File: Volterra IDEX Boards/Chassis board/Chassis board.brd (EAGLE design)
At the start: 102.2 x 54 mm, 29 parts, among them K1 FFC/FPC/34PIN/1MMPITCH/TOPLOCK, K2 FFC/FPC/34PIN/1MMPITCH/TOPLOCK, K3 FFC/FPC/34PIN/1MMPITCH/TOPLOCK, X1 JST-XH-02-PIN-LONG-PAD

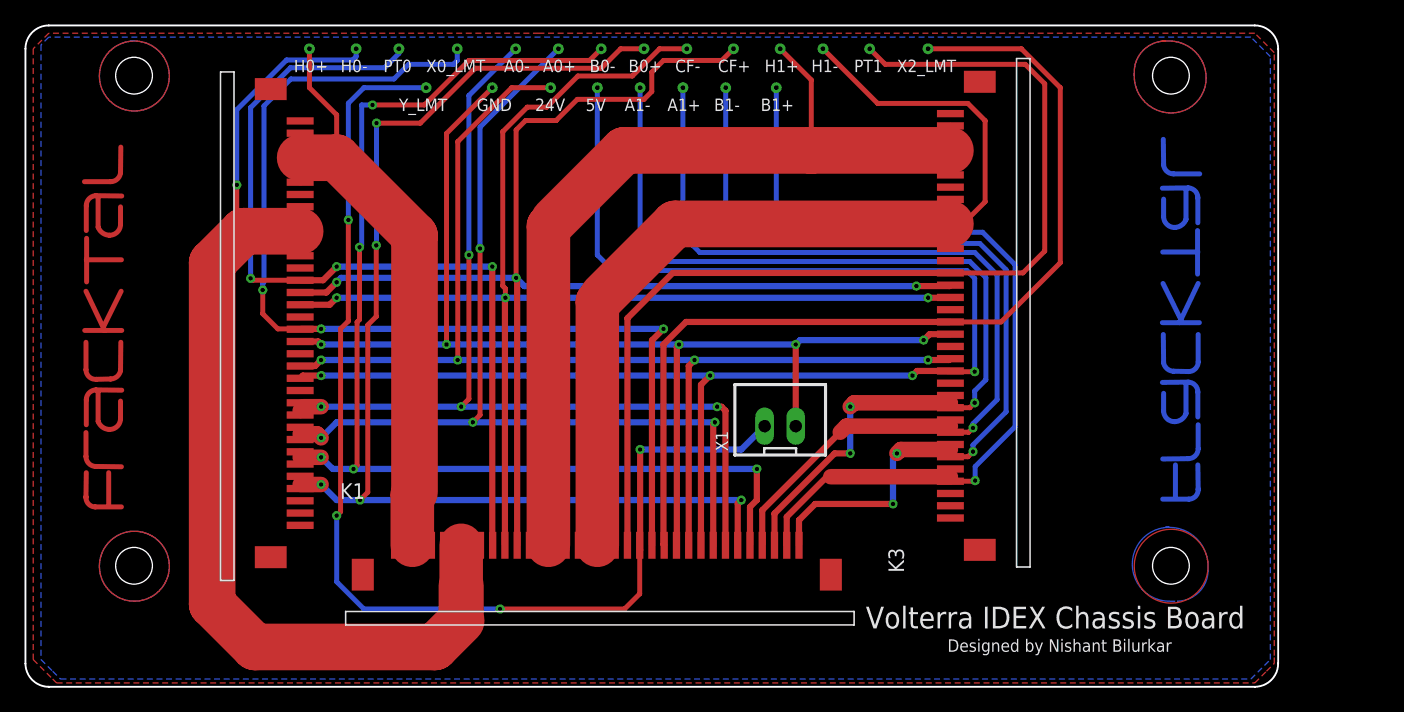
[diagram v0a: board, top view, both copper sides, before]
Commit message: DRC checked of Chassis, Carriage 1 & 2, and created CAM files
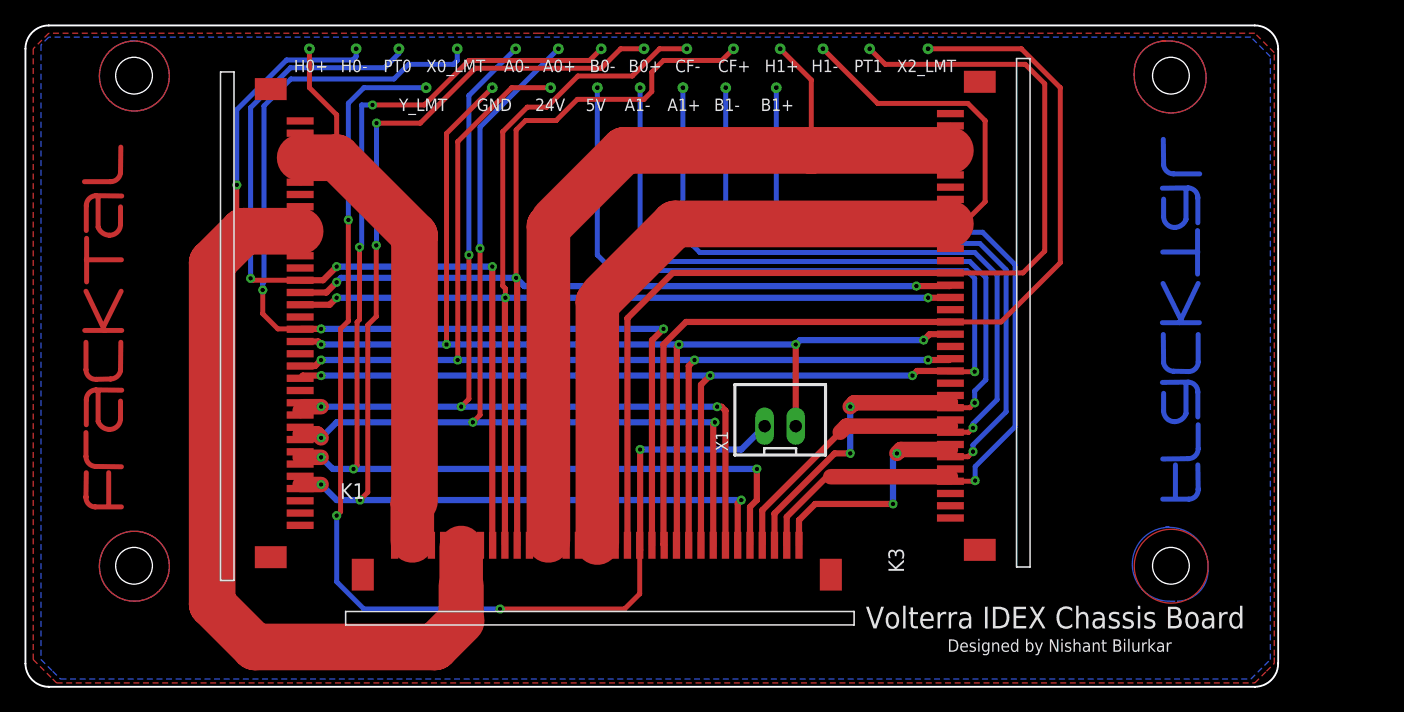
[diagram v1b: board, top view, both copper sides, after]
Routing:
- net H0+: track 53.9 -> 55.4 mm
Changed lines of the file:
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@@
 <contactref element="K2" pad="6"/>
 <contactref element="TP21" pad="P$1"/>
-<wire x1="37.7505" y1="15.3595" x2="38.7505" y2="15.3595" width="0.1524" layer="1"/>
-<wire x1="38.7505" y1="15.3595" x2="39.1922" y2="15.3595" width="0.1524" layer="1"/>
-<wire x1="39.37" y1="15.3595" x2="39.7505" y2="15.3595" width="0.1524" layer="1"/>
-<wire x1="39.7505" y1="15.3595" x2="40.7505" y2="15.3595" width="0.1524" layer="1"/>
-<wire x1="39.1922" y1="19.5072" x2="39.37" y2="19.685" width="3.556" layer="1"/>
-<wire x1="39.1922" y1="19.5072" x2="39.1922" y2="15.3595" width="3.556" layer="1"/>
-<wire x1="39.37" y1="19.685" x2="39.37" y2="40.64" width="3.81" layer="1"/>
+<wire x1="39.1922" y1="18.796" x2="39.37" y2="18.9738" width="3.556" layer="1"/>
+<wire x1="39.1922" y1="15.7151" x2="39.1922" y2="18.796" width="3.556" layer="1"/>
+<wire x1="39.37" y1="18.9738" x2="39.37" y2="40.64" width="3.81" layer="1"/>
 <wire x1="30.04" y1="46.99" x2="33.02" y2="46.99" width="3.81" layer="1"/>
 <wire x1="39.37" y1="40.64" x2="33.02" y2="46.99" width="3.81" layer="1"/>
@@
 <wire x1="30.04" y1="46.99" x2="30.04" y2="45.99" width="0.508" layer="1"/>
 <wire x1="30.04" y1="45.99" x2="30.04" y2="44.99" width="0.508" layer="1"/>
+<wire x1="40.7505" y1="15.3595" x2="39.7505" y2="15.3595" width="0.2032" layer="1"/>
+<wire x1="37.7505" y1="15.3595" x2="38.7505" y2="15.3595" width="0.2032" layer="1"/>
+<wire x1="38.7505" y1="15.3595" x2="39.7505" y2="15.3595" width="0.2032" layer="1"/>
+<wire x1="37.7505" y1="15.3595" x2="38.1061" y2="15.7151" width="0.2032" layer="1"/>
+<wire x1="38.1061" y1="15.7151" x2="39.1922" y2="15.7151" width="0.2032" layer="1"/>
 </signal>
 <signal name="H0-">
@@
 <contactref element="K2" pad="11"/>
 <contactref element="TP1" pad="P$1"/>
-<wire x1="41.7505" y1="15.3595" x2="42.7505" y2="15.3595" width="0.1524" layer="1"/>
-<wire x1="43.7505" y1="15.3595" x2="43.18" y2="15.3595" width="0.1524" layer="1"/>
-<wire x1="42.7505" y1="15.3595" x2="43.18" y2="15.3595" width="0.1524" layer="1"/>
-<wire x1="43.7505" y1="15.3595" x2="44.7505" y2="15.3595" width="0.1524" layer="1"/>
-<wire x1="43.18" y1="15.3595" x2="43.18" y2="12.065" width="3.556" layer="1"/>
+<wire x1="43.18" y1="12.065" x2="43.18" y2="15.1817" width="3.556" layer="1"/>
 <wire x1="43.18" y1="12.065" x2="43.18" y2="9.2075" width="3.683" layer="1"/>
 <wire x1="43.18" y1="9.2075" x2="41.0337" y2="7.0612" width="3.81" layer="1"/>
@@
 <wire x1="30.04" y1="40.99" x2="30.04" y2="39.99" width="1.27" layer="1"/>
 <wire x1="30.04" y1="41.99" x2="30.04" y2="42.99" width="0.508" layer="1"/>
-<wire x1="30.04" y1="39.99" x2="30.04" y2="38.99" width="0.1524" layer="1"/>
 <wire x1="25.4325" y1="40.99" x2="24.8666" y2="41.5559" width="0.4064" layer="1"/>
 <wire x1="24.8666" y1="41.5559" x2="24.8666" y2="44.7675" width="0.4064" layer="1"/>
@@
 <wire x1="34.3281" y1="54.9656" x2="34.6075" y2="55.245" width="0.4064" layer="16"/>
 <wire x1="34.6075" y1="55.245" x2="34.6075" y2="55.88" width="0.4064" layer="16"/>
+<wire x1="41.7505" y1="15.3595" x2="42.7505" y2="15.3595" width="0.2032" layer="1"/>
+<wire x1="42.7505" y1="15.3595" x2="43.7505" y2="15.3595" width="0.2032" layer="1"/>
+<wire x1="43.7505" y1="15.3595" x2="44.7505" y2="15.3595" width="0.2032" layer="1"/>
+<wire x1="43.18" y1="15.1817" x2="43.3578" y2="15.3595" width="0.2032" layer="1"/>
+<wire x1="43.3578" y1="15.3595" x2="43.7505" y2="15.3595" width="0.2032" layer="1"/>
+<wire x1="30.04" y1="39.99" x2="30.04" y2="38.99" width="0.2032" layer="1"/>
 </signal>
 <signal name="PT0">
@@
 <contactref element="K3" pad="29"/>
 <contactref element="TP22" pad="P$1"/>
-<wire x1="48.7505" y1="15.3595" x2="49.7505" y2="15.3595" width="0.1524" layer="1"/>
-<wire x1="49.7505" y1="15.3595" x2="50.2984" y2="15.3595" width="0.1524" layer="1"/>
-<wire x1="50.2984" y1="15.3595" x2="50.7505" y2="15.3595" width="0.1524" layer="1"/>
-<wire x1="50.7505" y1="15.3595" x2="51.7505" y2="15.3595" width="0.1524" layer="1"/>
 <wire x1="83.107" y1="47.587" x2="71.755" y2="47.587" width="3.81" layer="1"/>
 <wire x1="71.755" y1="47.587" x2="56.477" y2="47.587" width="3.81" layer="1"/>
@@
 <wire x1="83.107" y1="47.587" x2="83.107" y2="46.587" width="1.27" layer="1"/>
 <wire x1="83.107" y1="48.587" x2="83.107" y2="49.587" width="0.508" layer="1"/>
-<wire x1="83.107" y1="46.587" x2="83.107" y2="45.587" width="0.1524" layer="1"/>
 <wire x1="69.215" y1="55.88" x2="71.755" y2="53.34" width="0.4064" layer="1"/>
 <wire x1="71.755" y1="53.34" x2="71.755" y2="47.587" width="0.4064" layer="1"/>
 <wire x1="50.7505" y1="41.8605" x2="50.2984" y2="41.4084" width="3.556" layer="1"/>
-<wire x1="50.2984" y1="41.4084" x2="50.2984" y2="15.3595" width="3.556" layer="1"/>
+<wire x1="50.2984" y1="41.4084" x2="50.2984" y2="15.7151" width="3.556" layer="1"/>
+<wire x1="48.7505" y1="15.3595" x2="49.7505" y2="15.3595" width="0.2032" layer="1"/>
+<wire x1="50.7505" y1="15.3595" x2="51.7505" y2="15.3595" width="0.2032" layer="1"/>
+<wire x1="50.7505" y1="15.3595" x2="49.7505" y2="15.3595" width="0.2032" layer="1"/>
+<wire x1="50.2984" y1="15.7151" x2="50.654" y2="15.3595" width="0.2032" layer="1"/>
+<wire x1="50.654" y1="15.3595" x2="50.7505" y2="15.3595" width="0.2032" layer="1"/>
+<wire x1="83.107" y1="46.587" x2="83.107" y2="45.587" width="0.2032" layer="1"/>
 </signal>
 <signal name="H1-">
@@
 <contactref element="K3" pad="23"/>
 <contactref element="TP10" pad="P$1"/>
-<wire x1="52.7505" y1="15.3595" x2="53.7505" y2="15.3595" width="0.1524" layer="1"/>
-<wire x1="53.7505" y1="15.3595" x2="54.2925" y2="15.3595" width="0.1524" layer="1"/>
-<wire x1="54.2925" y1="15.3595" x2="54.7505" y2="15.3595" width="0.1524" layer="1"/>
-<wire x1="54.7505" y1="15.3595" x2="55.7505" y2="15.3595" width="0.1524" layer="1"/>
 <wire x1="60.637" y1="41.587" x2="83.107" y2="41.587" width="3.81" layer="1"/>
 <wire x1="60.637" y1="41.587" x2="54.7505" y2="35.7005" width="3.81" layer="1"/>
-<wire x1="83.107" y1="39.587" x2="83.107" y2="40.587" width="0.1524" layer="1"/>
-<wire x1="83.107" y1="40.587" x2="83.107" y2="41.587" width="0.1524" layer="1"/>
-<wire x1="83.107" y1="41.587" x2="83.107" y2="42.587" width="0.1524" layer="1"/>
-<wire x1="83.107" y1="42.587" x2="83.107" y2="43.587" width="0.1524" layer="1"/>
 <wire x1="54.7505" y1="35.7005" x2="54.2925" y2="35.2425" width="3.556" layer="1"/>
-<wire x1="54.2925" y1="35.2425" x2="54.2925" y2="15.3595" width="3.556" layer="1"/>
+<wire x1="54.2925" y1="35.2425" x2="54.2925" y2="15.5373" width="3.556" layer="1"/>
 <wire x1="72.7075" y1="55.88" x2="77.1671" y2="51.4204" width="0.4064" layer="1"/>
 <wire x1="77.1671" y1="51.4204" x2="84.53209375" y2="51.4204" width="0.4064" layer="1"/>
@@
 <wire x1="85.9409" y1="43.3959" x2="84.132" y2="41.587" width="0.4064" layer="1"/>
 <wire x1="84.132" y1="41.587" x2="83.107" y2="41.587" width="0.4064" layer="1"/>
+<wire x1="52.7505" y1="15.3595" x2="53.7505" y2="15.3595" width="0.2032" layer="1"/>
+<wire x1="53.7505" y1="15.3595" x2="54.7505" y2="15.3595" width="0.2032" layer="1"/>
+<wire x1="55.7505" y1="15.3595" x2="54.7505" y2="15.3595" width="0.2032" layer="1"/>
+<wire x1="54.2925" y1="15.5373" x2="54.4703" y2="15.3595" width="0.2032" layer="1"/>
+<wire x1="54.4703" y1="15.3595" x2="54.7505" y2="15.3595" width="0.2032" layer="1"/>
+<wire x1="83.107" y1="43.587" x2="83.107" y2="42.587" width="0.2032" layer="1"/>
+<wire x1="83.107" y1="42.587" x2="83.107" y2="41.587" width="0.2032" layer="1"/>
+<wire x1="83.107" y1="41.587" x2="83.107" y2="40.587" width="0.2032" layer="1"/>
+<wire x1="83.107" y1="40.587" x2="83.107" y2="39.587" width="0.2032" layer="1"/>
 </signal>
 <signal name="PT1">
@@
 <contactref element="K3" pad="10"/>
 <contactref element="TP14" pad="P$1"/>
-<wire x1="83.107" y1="26.67" x2="83.107" y2="26.587" width="0.1524" layer="1"/>
 <wire x1="68.7505" y1="15.3595" x2="68.7505" y2="17.9505" width="0.508" layer="1"/>
 <wire x1="73.66" y1="22.86" x2="68.7505" y2="17.9505" width="0.508" layer="1"/>
@@
 <wire x1="84.6895" y1="26.587" x2="83.107" y2="26.587" width="0.4064" layer="1"/>
 <wire x1="57.785" y1="40.64" x2="59.9059" y2="38.5191" width="0.4064" layer="16"/>
-<wire x1="83.107" y1="27.587" x2="83.107" y2="26.9875" width="0.4064" layer="1"/>
-<wire x1="83.107" y1="26.9875" x2="83.107" y2="26.67" width="0.4064" layer="1"/>
-<wire x1="83.107" y1="26.9875" x2="75.2475" y2="26.9875" width="1.27" layer="1"/>
-<wire x1="75.2475" y1="26.9875" x2="74.93" y2="26.67" width="1.27" layer="1"/>
+<wire x1="74.93" y1="26.67" x2="75.2475" y2="26.9875" width="1.27" layer="1"/>
+<wire x1="83.107" y1="27.587" x2="83.107" y2="27.0256" width="0.2032" layer="1"/>
+<wire x1="83.107" y1="27.0256" x2="83.107" y2="26.587" width="0.2032" layer="1"/>
+<wire x1="83.0689" y1="26.9875" x2="83.107" y2="27.0256" width="1.27" layer="1"/>
+<wire x1="75.2475" y1="26.9875" x2="83.0689" y2="26.9875" width="1.27" layer="1"/>
 </signal>
 <signal name="B1+">
